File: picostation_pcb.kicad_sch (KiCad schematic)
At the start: 13 parts, among them J1 Conn_01x06_Female, J2 Conn_01x20_Female, J3 PICO, J4 Conn_01x20_Female, U1 LM78M05_TO252

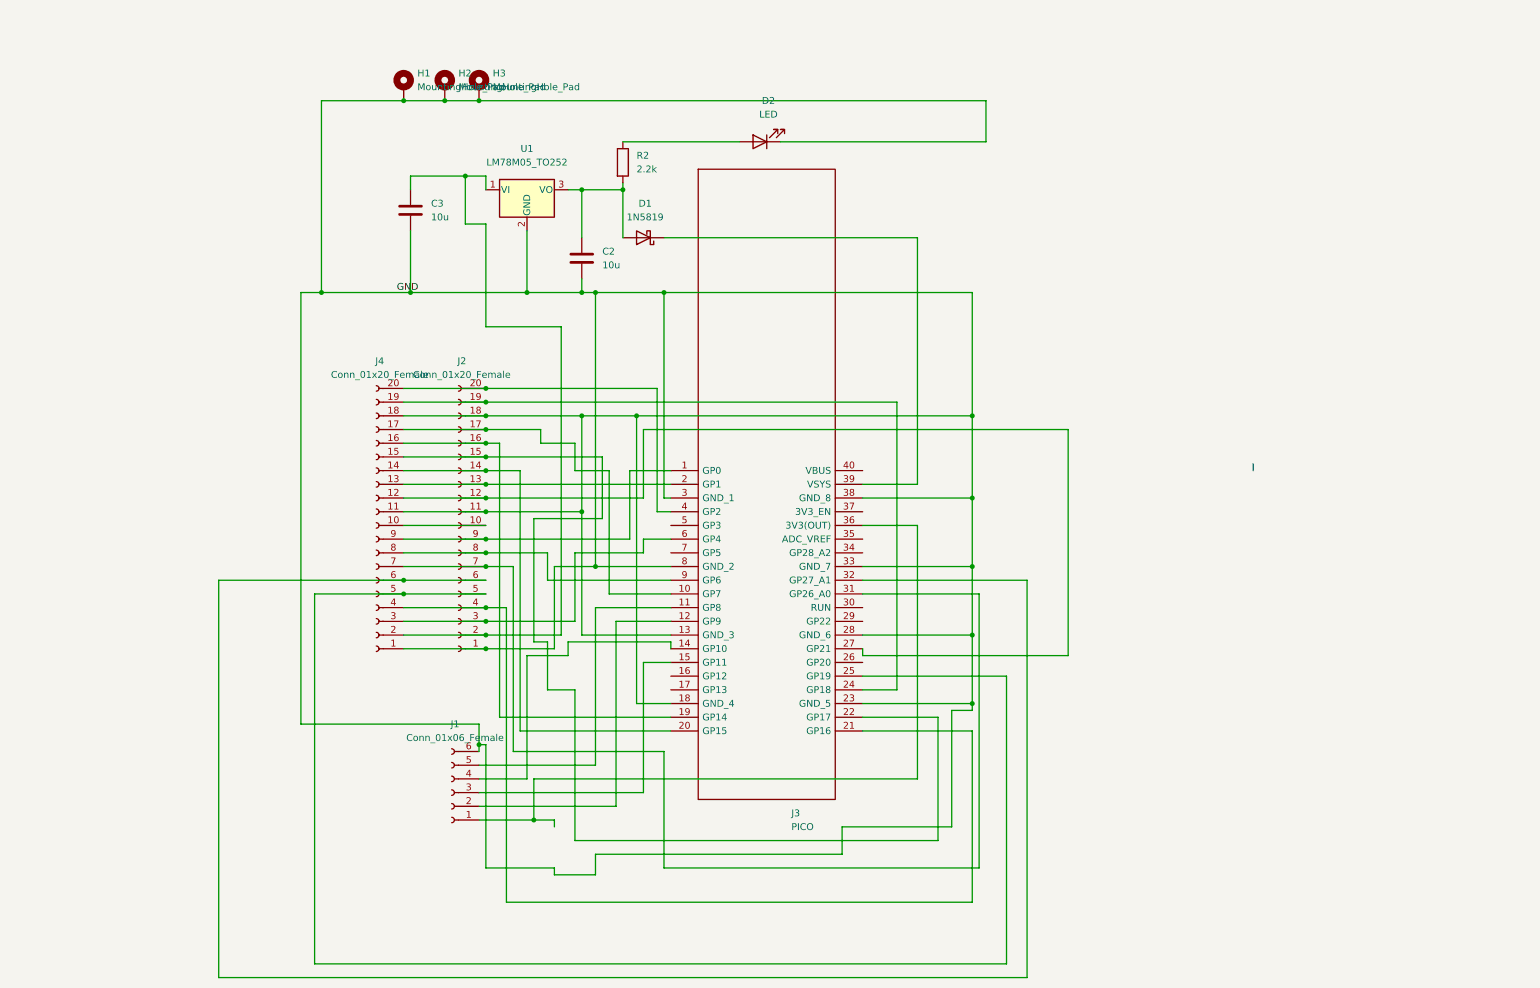
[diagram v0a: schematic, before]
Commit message: updated PCB
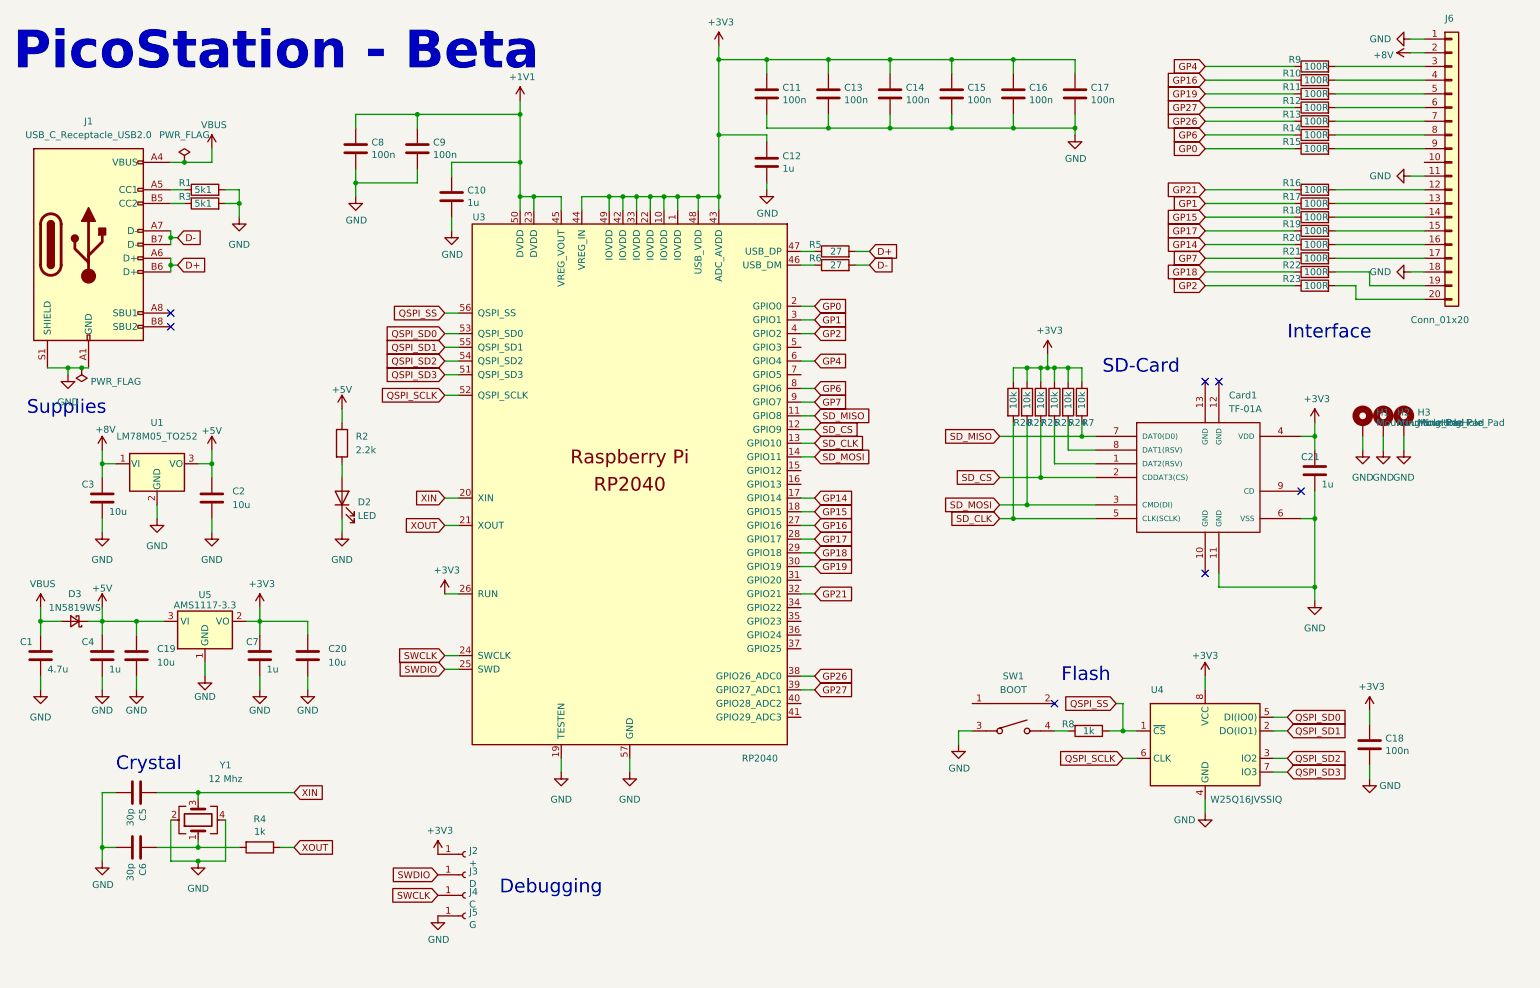
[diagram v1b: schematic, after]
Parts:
- removed D1: 1N5819, Diode_SMD:D_SOD-123, symbol Diode:1N5819
- removed J1: Conn_01x06_Female, paulo:SD, symbol Connector:Conn_01x06_Female
- removed J2: Conn_01x20_Female, Connector_FFC-FPC:TE_2-84952-0_1x20-1MP_P1.0mm_Horizontal, symbol Connector:Conn_01x20_Female
- removed J3: PICO, PICO:PICO, symbol pico:PICO
- removed J4: Conn_01x20_Female, Connector_PinSocket_2.54mm:PinSocket_2x10_P2.54mm_Vertical, symbol Connector:Conn_01x20_Female
- added C1: 4.7u, Capacitor_SMD:C_0603_1608Metric_Pad1.08x0.95mm_HandSolder, symbol Device:C
- added C10, C12, C21, C4, C7: 1u, Capacitor_SMD:C_0603_1608Metric_Pad1.08x0.95mm_HandSolder, symbol Device:C
- added C11, C13, C14, C15, C16, C17, C18, C8, C9: 100n, Capacitor_SMD:C_0603_1608Metric_Pad1.08x0.95mm_HandSolder, symbol Device:C
- added C19, C20: 10u, Capacitor_SMD:C_0805_2012Metric_Pad1.18x1.45mm_HandSolder, symbol Device:C
- added C5, C6: 30p, Capacitor_SMD:C_0603_1608Metric_Pad1.08x0.95mm_HandSolder, symbol Device:C
- added Card1: TF-01A, kicad_lceda:TF-SMD_TF-01A, symbol kicad_lceda:TF-01A
- added D3: 1N5819WS, Diode_SMD:D_SOD-323, symbol Device:D_Schottky_Small
- added J1: USB_C_Receptacle_USB2.0, Connector_USB:USB_C_Receptacle_HRO_TYPE-C-31-M-12, symbol Connector:USB_C_Receptacle_USB2.0
- added J2: +, TestPoint:TestPoint_Pad_D1.5mm, symbol Connector:Conn_01x01_Female
- added J3: D, TestPoint:TestPoint_Pad_D1.5mm, symbol Connector:Conn_01x01_Female
- added J4: C, TestPoint:TestPoint_Pad_D1.5mm, symbol Connector:Conn_01x01_Female
- added J5: G, TestPoint:TestPoint_Pad_D1.5mm, symbol Connector:Conn_01x01_Female
- added J6: Conn_01x20, Connector_FFC-FPC:Molex_200528-0200_1x20-1MP_P1.00mm_Horizontal, symbol Connector_Generic:Conn_01x20
- added R1, R3: 5k1, Resistor_SMD:R_0603_1608Metric_Pad0.98x0.95mm_HandSolder, symbol Device:R
- added R10, R11, R12, R13, R14, R15, R16, R17, R18, R19, R20, R21, R22, R23, R9: 100R, Resistor_SMD:R_0603_1608Metric_Pad0.98x0.95mm_HandSolder, symbol Device:R
- added R24, R25, R26, R27, R28, R7: 10k, Resistor_SMD:R_0603_1608Metric_Pad0.98x0.95mm_HandSolder, symbol Device:R
- added R4, R8: 1k, Resistor_SMD:R_0603_1608Metric_Pad0.98x0.95mm_HandSolder, symbol Device:R
- added R5, R6: 27, Resistor_SMD:R_0603_1608Metric_Pad0.98x0.95mm_HandSolder, symbol Device:R
- added SW1: BOOT, kicad_lceda:SW-SMD_TS24CA, symbol kicad_lceda:TS24CA
- added U3: RP2040, RP2040_minimal:RP2040-QFN-56, symbol MCU_RaspberryPi_RP2040:RP2040
- added U4: W25Q16JVSSIQ, Package_SO:SOIC-8_5.23x5.23mm_P1.27mm, symbol Memory_Flash:W25Q128JVS
- added U5: AMS1117-3.3, Package_TO_SOT_SMD:SOT-223-3_TabPin2, symbol Regulator_Linear:AMS1117-3.3
- added Y1: 12 Mhz, Crystal:Crystal_SMD_3225-4Pin_3.2x2.5mm, symbol Device:Crystal_GND24
- H1, H2, H3: footprint MountingHole:MountingHole_2.5mm_Pad -> MountingHole:MountingHole_2.2mm_M2_DIN965_Pad
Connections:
- net GND: now also C1.1, C10.2, C11.2, C12.2, C13.2, C14.2, C15.2, C16.2, C17.2, C18.2, C19.2, C20.2, C21.2, C4.2, C5.2, C6.2, C7.2, C8.2, C9.2, Card1.11 (GND), Card1.6 (VSS), J1.A1 (GND), J1.A12 (GND), J1.B1 (GND), J1.B12 (GND), J1.S1 (SHIELD), J5.1 (Pin_1), J6.1 (Pin_1), J6.11 (Pin_11), J6.18 (Pin_18), R1.2, R3.2, SW1.3, U3.19 (TESTEN), U3.57 (GND), U4.4 (GND), U5.1 (GND), Y1.2, Y1.4
- net +5V: now reaches C2.1, U1.3 (VO)
- net +5V: now also R2.1, C19.1, C4.1, D3.1 (K), U5.3 (VI); no longer R2.2
- net at D2.2 (A): now also R2.2; no longer R2.1
- net +8V: now reaches C3.1, U1.1 (VI)
- net +8V: now also J6.2 (Pin_2)
- new net: J6.9 (Pin_9), R15.2
- new net: J6.13 (Pin_13), R17.2
- new net: J1.B5 (CC2), R3.1
- new net: J6.19 (Pin_19), R22.2
- new net: J6.8 (Pin_8), R14.2
- new net: C6.1, R4.2, Y1.1
- new net: J6.17 (Pin_17), R21.2
- new net: R8.2, SW1.4
- new net: J1.A5 (CC1), R1.1
- new net: R6.1, U3.46 (USB_DM)
- new net: J6.5 (Pin_5), R11.2
- new net: J6.3 (Pin_3), R9.2
- new net: J6.14 (Pin_14), R18.2
- new net: J6.6 (Pin_6), R12.2
- new net: R5.1, U3.47 (USB_DP)
- new net: Card1.1 (DAT2(RSV)), R25.2
- new net: Card1.8 (DAT1(RSV)), R24.2
- new net: J6.12 (Pin_12), R16.2
- new net: J6.7 (Pin_7), R13.2
- new net: J6.16 (Pin_16), R20.2
- new net: J6.15 (Pin_15), R19.2
- new net: J6.20 (Pin_20), R23.2
- new net: J6.4 (Pin_4), R10.2
- new net +1V1: C10.1, C8.1, C9.1, U3.23 (DVDD), U3.45 (VREG_VOUT), U3.50 (DVDD)
- new net +3V3: C11.1, C12.1, C13.1, C14.1, C15.1, C16.1, C17.1, C18.1, C20.1, C21.1, C7.1, Card1.4 (VDD), J2.1 (Pin_1), R24.1, R25.1, R26.1, R27.1, R28.1, R7.1, U3.1 (IOVDD), U3.10 (IOVDD), U3.22 (IOVDD), U3.26 (RUN), U3.33 (IOVDD), U3.42 (IOVDD), U3.43 (ADC_AVDD), U3.44 (VREG_IN), U3.48 (USB_VDD), U3.49 (IOVDD), U4.8 (VCC), U5.2 (VO)
- new net D+: J1.A6 (D+), J1.B6 (D+), R5.2
- new net D-: J1.A7 (D-), J1.B7 (D-), R6.2
- new net GP0: R15.1, U3.2 (GPIO0)
- new net GP1: R17.1, U3.3 (GPIO1)
- new net GP14: R20.1, U3.17 (GPIO14)
- new net GP15: R18.1, U3.18 (GPIO15)
- new net GP16: R10.1, U3.27 (GPIO16)
- new net GP17: R19.1, U3.28 (GPIO17)
- new net GP18: R22.1, U3.29 (GPIO18)
- new net GP19: R11.1, U3.30 (GPIO19)
- new net GP2: R23.1, U3.4 (GPIO2)
- new net GP21: R16.1, U3.32 (GPIO21)
- new net GP26: R13.1, U3.38 (GPIO26_ADC0)
- new net GP27: R12.1, U3.39 (GPIO27_ADC1)
- new net GP4: R9.1, U3.6 (GPIO4)
- new net GP6: R14.1, U3.8 (GPIO6)
- new net GP7: R21.1, U3.9 (GPIO7)
- new net QSPI_SCLK: U3.52 (QSPI_SCLK), U4.6 (CLK)
- new net QSPI_SD0: U3.53 (QSPI_SD0), U4.5 (DI(IO0))
- new net QSPI_SD1: U3.55 (QSPI_SD1), U4.2 (DO(IO1))
- new net QSPI_SD2: U3.54 (QSPI_SD2), U4.3 (IO2)
- new net QSPI_SD3: U3.51 (QSPI_SD3), U4.7 (IO3)
- new net QSPI_SS: R8.1, U3.56 (QSPI_SS), U4.1 (~{CS})
- new net SD_CLK: Card1.5 (CLK(SCLK)), R28.2, U3.13 (GPIO10)
- new net SD_CS: Card1.2 (CDDAT3(CS)), R26.2, U3.12 (GPIO9)
- new net SD_MISO: Card1.7 (DAT0(D0)), R7.2, U3.11 (GPIO8)
- new net SD_MOSI: Card1.3 (CMD(DI)), R27.2, U3.14 (GPIO11)
- new net SWCLK: J4.1 (Pin_1), U3.24 (SWCLK)
- new net SWDIO: J3.1 (Pin_1), U3.25 (SWD)
- new net VBUS: C1.2, D3.2 (A), J1.A4 (VBUS), J1.A9 (VBUS), J1.B4 (VBUS), J1.B9 (VBUS)
- new net XIN: C5.1, U3.20 (XIN), Y1.3
- new net XOUT: R4.1, U3.21 (XOUT)
- no-connect marks 0 -> 7
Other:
- note added: "Crystal"
- note added: "Debugging"
- note added: "Flash"
- note added: "Interface"
- note added: "PicoStation - Beta"
- note added: "SD-Card"
- note added: "Supplies"
- moved on the sheet: C2, C3, D2, R2, U1
